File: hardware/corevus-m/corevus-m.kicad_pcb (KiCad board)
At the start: 2 copper layers, 90 x 40 mm, 88 parts, among them J1 Power In, J2 USB 2.0, J3 XH, J4 XH, SW1 BOOT, SW2 RST, T1 V_{SA}, T10 Gnd, T11 Step, T12 Diag, T13 CS, T14 En, T15 Dir, T16 Gnd, T17 Step, T18 Diag, T19 V_{SA}, T2 SClk, T20 SClk, T21 MOSI, T22 Gnd, T23 MISO, T24 3.3V, T25 CS, T26 En, T27 Dir, T28 Gnd, T29 Step, T3 MOSI, T30 Diag, T31 CS, T32 En, T33 Dir, T34 Gnd, T35 Step, T36 Diag, T4 Gnd, T5 MISO, T6 3.3V, T7 CS, T8 En, T9 Dir, U1 STM32G431CBUx, U2 TPS61040DBV, U3 XC6206P332MR, Y1 12 MHz

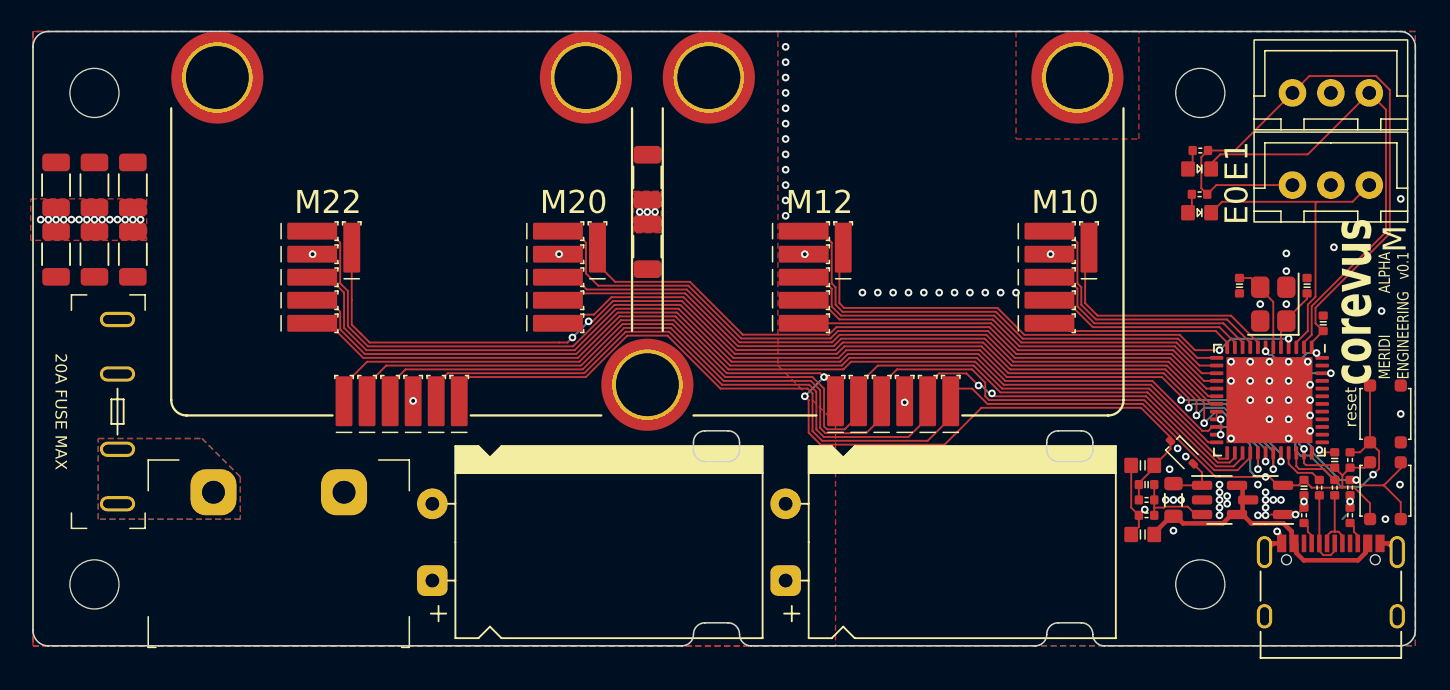
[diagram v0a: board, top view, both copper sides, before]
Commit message: test
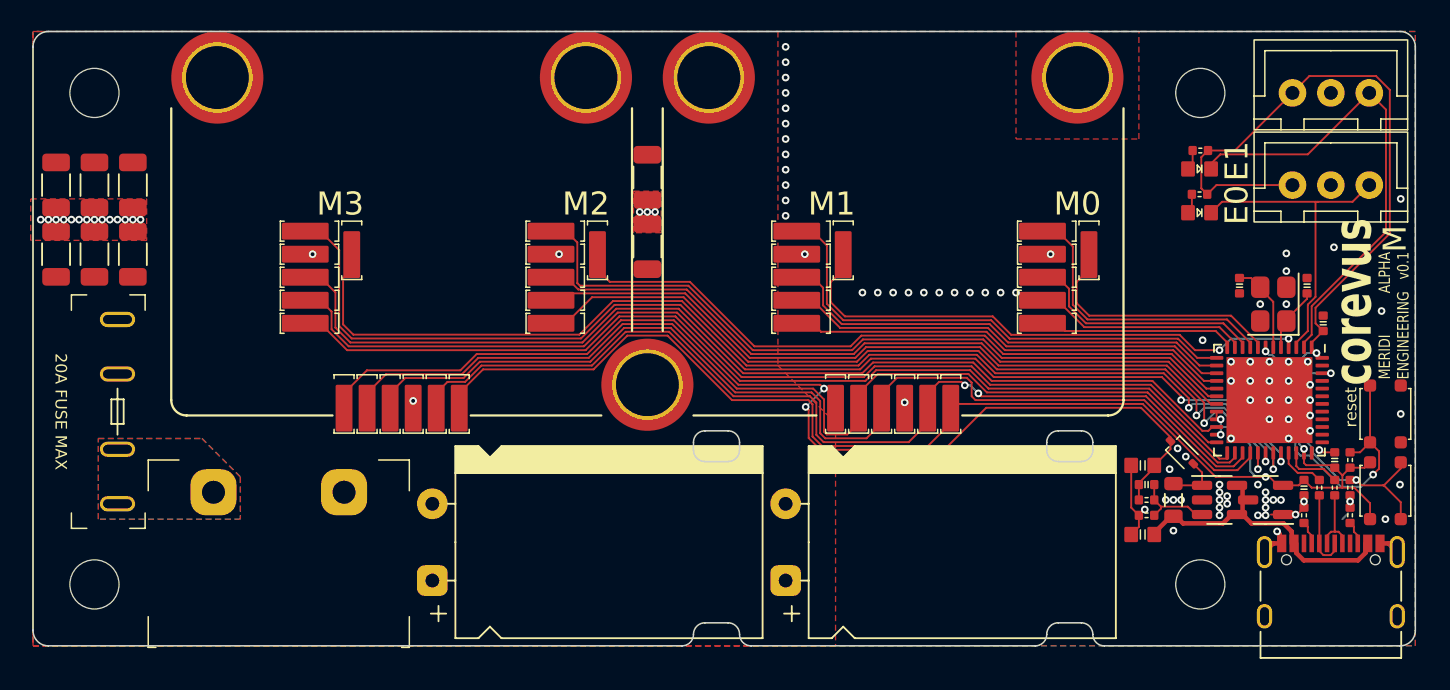
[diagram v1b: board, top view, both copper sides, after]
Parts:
- R7: value AkΩ -> 10kΩ
- R8: value AkΩ -> 100kΩ
- turned R10 to 90 degrees
- turned R9 to 90 degrees
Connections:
- R10 pad 1: Net-(U1-PA12) -> Net-(J2-D+-PadA6)
- R10 pad 2: Net-(J2-D+-PadA6) -> Net-(U1-PA12)
- R9 pad 1: Net-(U1-PA11) -> Net-(J2-D--PadA7)
- R9 pad 2: Net-(J2-D--PadA7) -> Net-(U1-PA11)
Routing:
- net /_{M12}Diag: track 35.9 -> 33.7 mm
- net /_{M12}~{CS}: track 27.6 -> 28.7 mm
- net /_{M10}Diag: track 17.2 -> 17.9 mm
- net /_{M20}Step: track 48.1 -> 48.8 mm
- net +3.3V: track 134.7 -> 135.5 mm
- net /MOSI: track 68.6 -> 68.0 mm
- net /SCK: track 68.6 -> 68.0 mm
- net /_{M22}Diag: track 74.7 -> 75.2 mm, vias 4 -> 2
- net GND: track 13.3 -> 13.0 mm, vias 104 -> 105
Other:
- board text added: "M0"
- board text added: "M1"
- board text added: "M2"
- board text added: "M3"
- board text removed: "M10"
- board text removed: "M12"
- board text removed: "M20"
- board text removed: "M22"
